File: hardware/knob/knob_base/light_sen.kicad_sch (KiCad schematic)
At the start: 7 parts, among them U1 LMV321

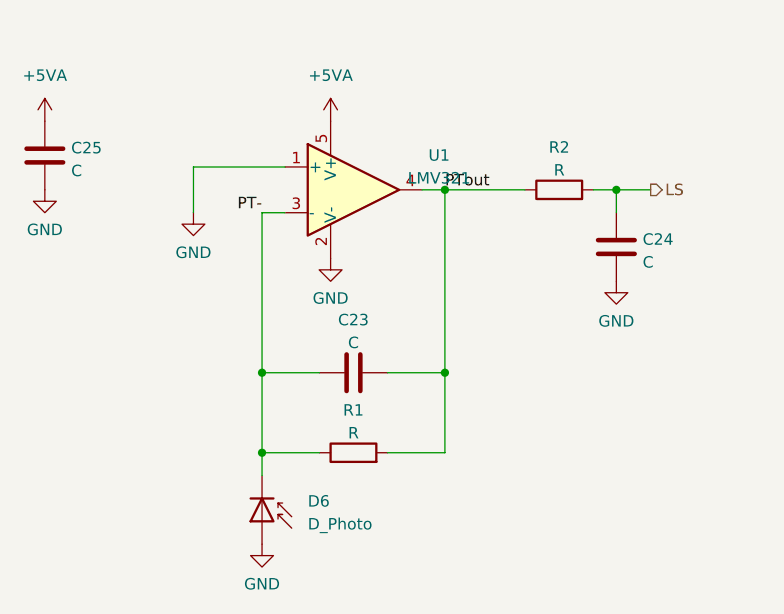
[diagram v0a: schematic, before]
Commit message: working
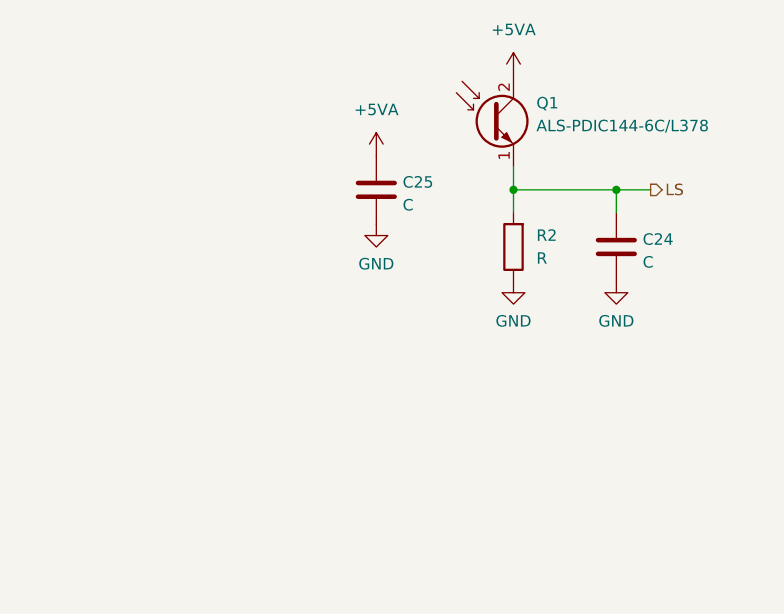
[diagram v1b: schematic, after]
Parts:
- removed C23: C, Capacitor_SMD:C_0603_1608Metric, symbol Device:C
- removed D6: D_Photo, LED_THT:LED_D3.0mm_Clear, symbol Device:D_Photo
- removed R1: R, Resistor_SMD:R_0603_1608Metric, symbol Device:R
- removed U1: LMV321, Package_TO_SOT_SMD:SOT-23-5, symbol Amplifier_Operational:LMV321
- added Q1: ALS-PDIC144-6C/L378, LED_THT:LED_D3.0mm_FlatTop, symbol Device:Q_Photo_NPN_EC
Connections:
- net PTout is gone; now on net GND: R2.1
- net +5VA: now also Q1.2 (C)
- net LS: now also Q1.1 (E)
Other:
- moved on the sheet: C25, R2
